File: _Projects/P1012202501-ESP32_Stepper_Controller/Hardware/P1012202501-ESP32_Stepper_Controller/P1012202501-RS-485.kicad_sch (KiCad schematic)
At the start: 5 parts, among them IC4 USP485REN-L_TR

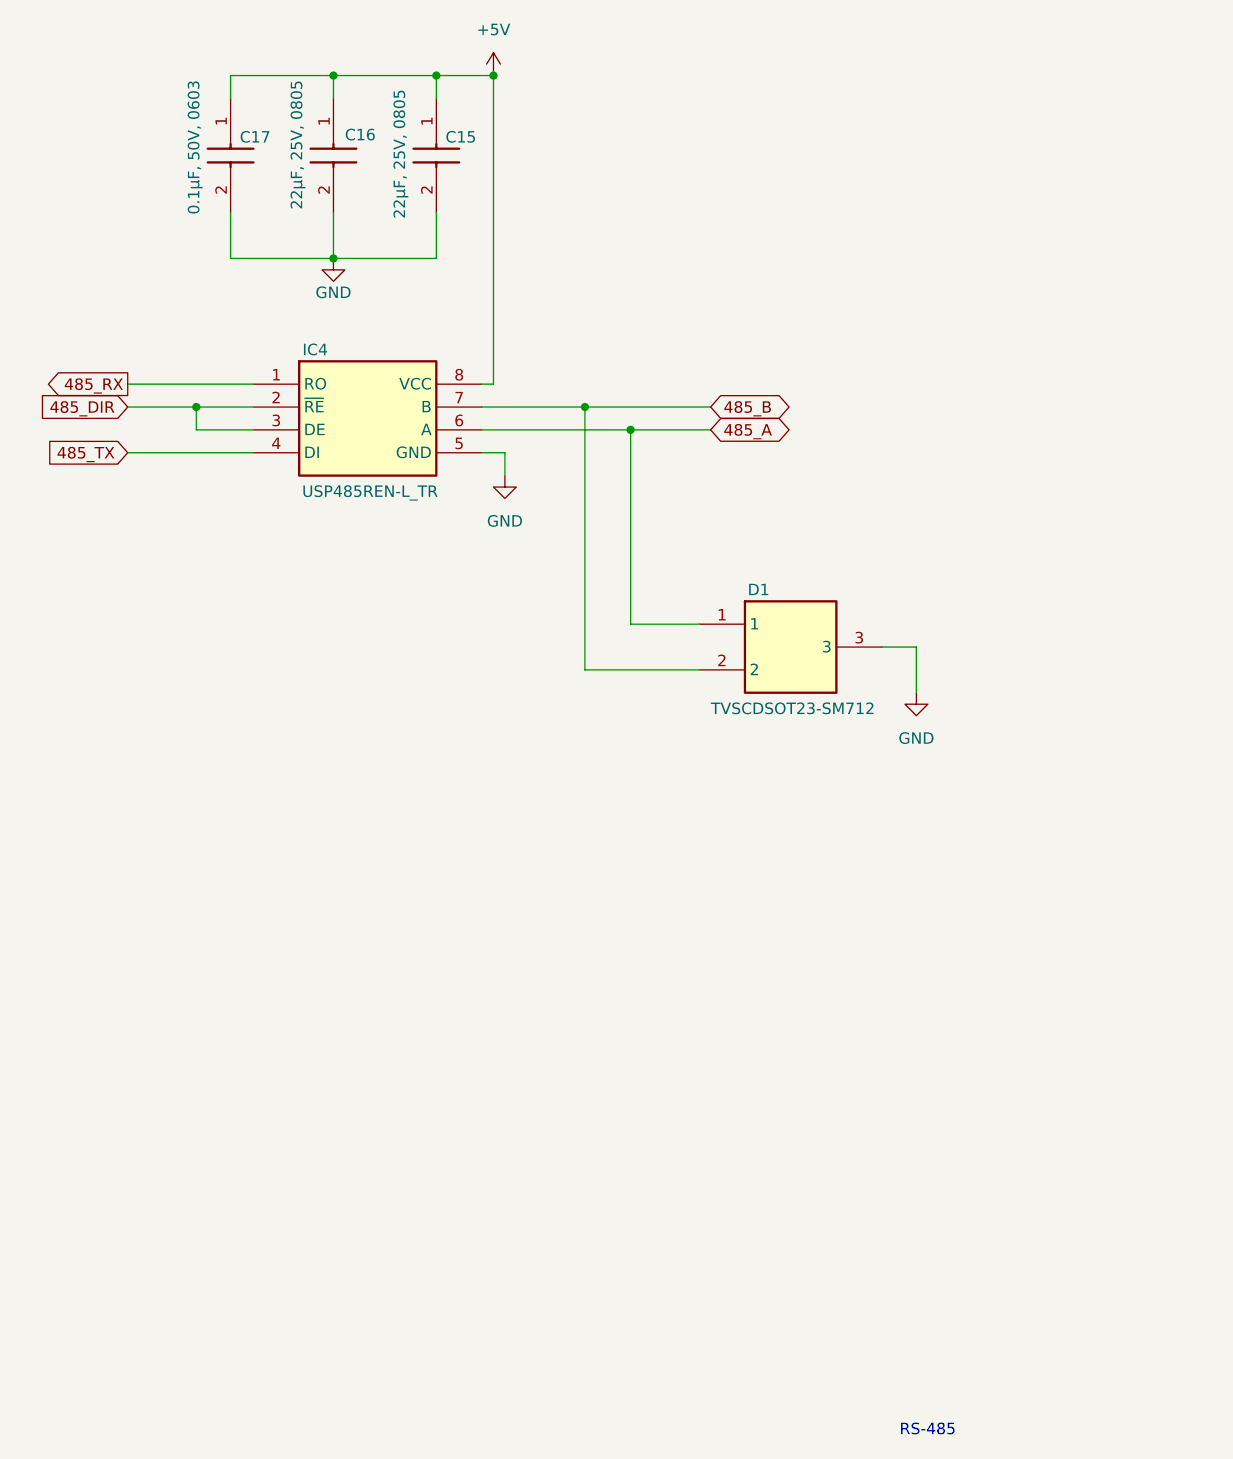
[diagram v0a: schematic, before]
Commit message: Added new content from stream.
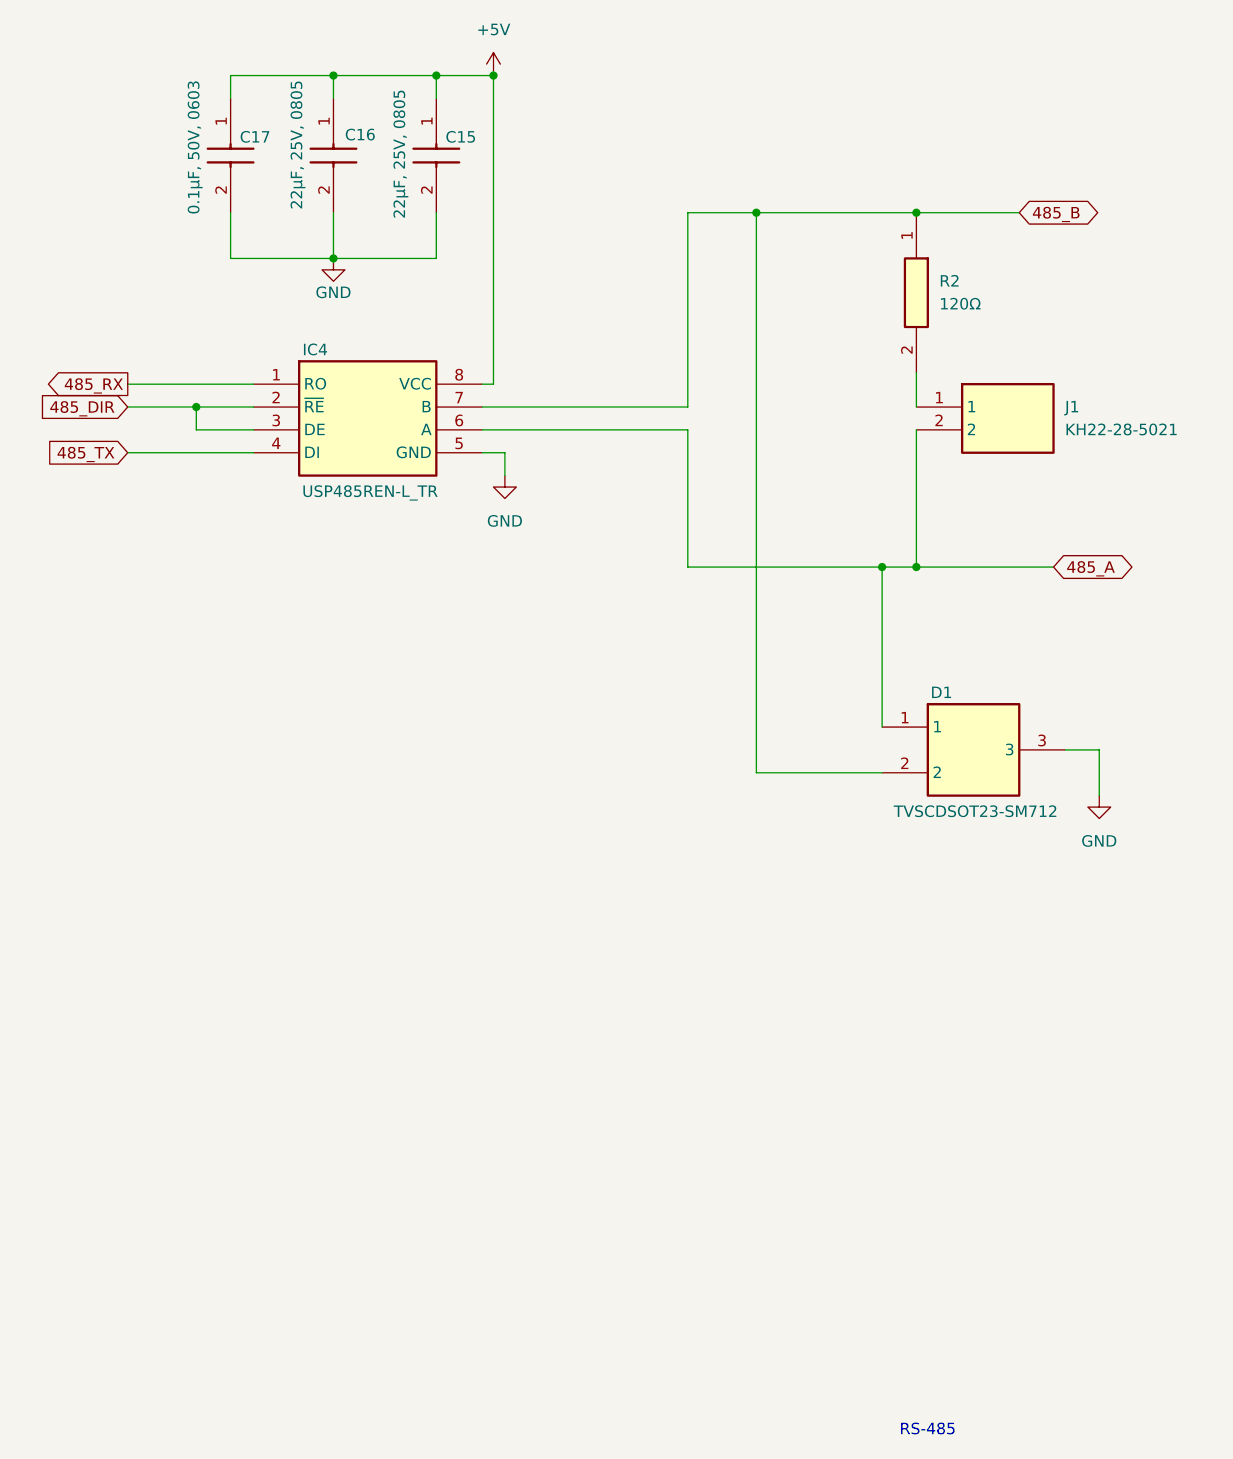
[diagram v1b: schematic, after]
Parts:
- added J1: KH22-28-5021, CONNECTORS:2x1HDR2.54mm, symbol CONNECTORS:KH22-28-5021
- added R2: RC0805121150AAB, COMPONENTS:RES-0805, symbol COMPONENTS:RC0805121150AAB
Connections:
- net 485_A: now also J1.2
- net 485_B: now also R2.1
- new net: J1.1, R2.2
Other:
- moved on the sheet: D1
